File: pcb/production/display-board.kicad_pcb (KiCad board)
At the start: 2 copper layers, 200 x 38.5 mm, 56 parts, among them J301 TO_MAIN, SW301 SAMPLE RATE, SW302 LOOPBACK, U301 HT1635D

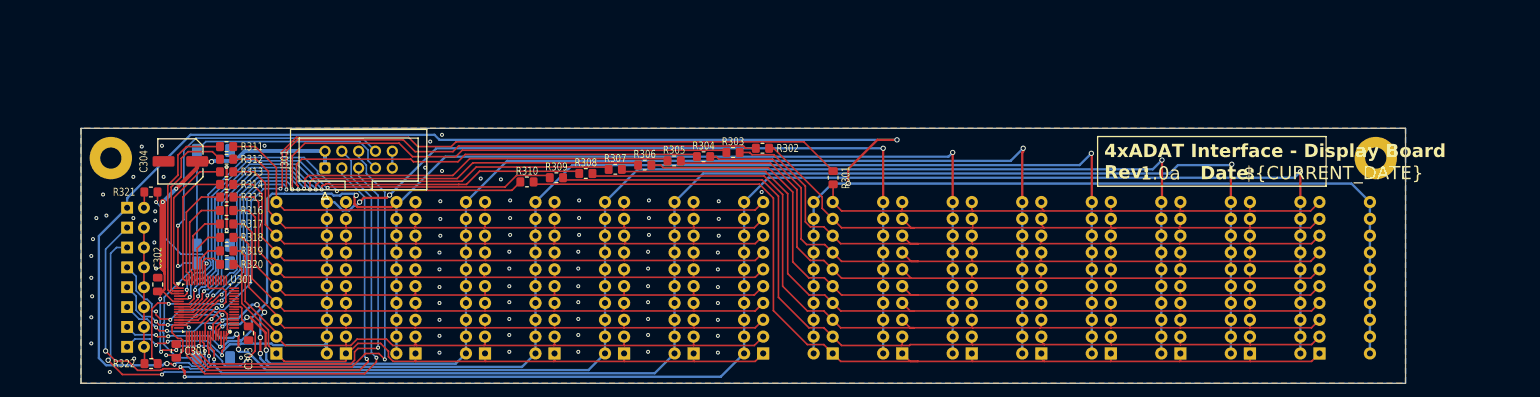
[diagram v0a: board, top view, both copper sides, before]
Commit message: Provide final rev 1.0a production files
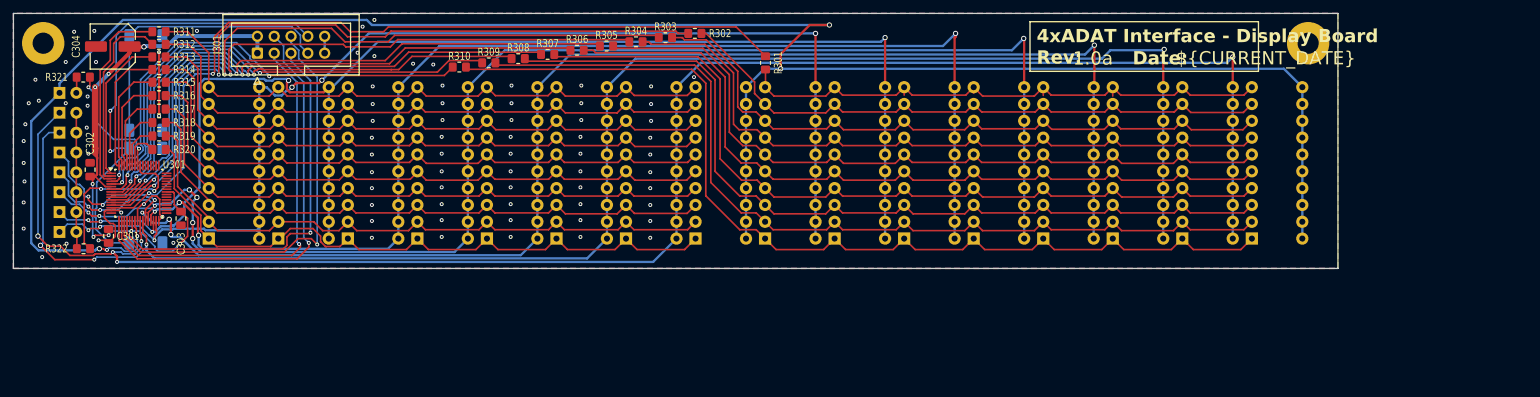
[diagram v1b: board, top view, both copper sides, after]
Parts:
- moved C301 20.1 mm to (37.0, 57.9)
- moved R303 20.1 mm to (121.1, 28.0)
- moved R322 20.1 mm to (33.2, 59.8)
- moved BAR301 20.1 mm to (213.5, 46.9)
- moved BAR302 20.1 mm to (203.0, 46.9)
- moved BAR303 20.1 mm to (192.5, 46.9)
- moved BAR304 20.1 mm to (182.0, 46.9)
- moved BAR305 20.1 mm to (171.5, 46.9)
- moved BAR306 20.1 mm to (161.0, 46.9)
- moved BAR307 20.1 mm to (150.5, 46.9)
- moved BAR308 20.1 mm to (140.0, 46.9)
- moved BAR309 20.1 mm to (129.5, 46.9)
- moved BAR310 20.1 mm to (119.0, 46.9)
- moved BAR311 20.1 mm to (108.5, 46.9)
- moved BAR312 20.1 mm to (98.0, 46.9)
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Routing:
- net /Display board/LED1: track 99.7 -> 95.7 mm
- net /Display board/LED3: track 113.5 -> 109.5 mm
- net /Display board/LED5: track 125.6 -> 121.9 mm
- net /Display board/LED18: track 100.2 -> 97.1 mm
- net /Display board/LED2: track 106.0 -> 103.3 mm
- net /Display board/LED4: track 118.2 -> 115.5 mm
- net /Display board/LED7: track 136.5 -> 134.2 mm
- net /Display board/LED11: track 96.7 -> 94.5 mm
- net /Display board/LED6: track 130.2 -> 128.1 mm
- net /Display board/LED15: track 98.4 -> 96.3 mm
- net /Display board/LED8: track 141.9 -> 140.4 mm
- net /Display board/LED16: track 97.6 -> 96.1 mm
- net /Display board/LED0: track 86.8 -> 88.1 mm
- net /Display board/LED13: track 96.7 -> 95.4 mm
- net /Display board/LED14: track 97.4 -> 96.2 mm
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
